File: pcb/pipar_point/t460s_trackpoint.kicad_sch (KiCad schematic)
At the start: 7 parts, among them X1 12.0 MHz

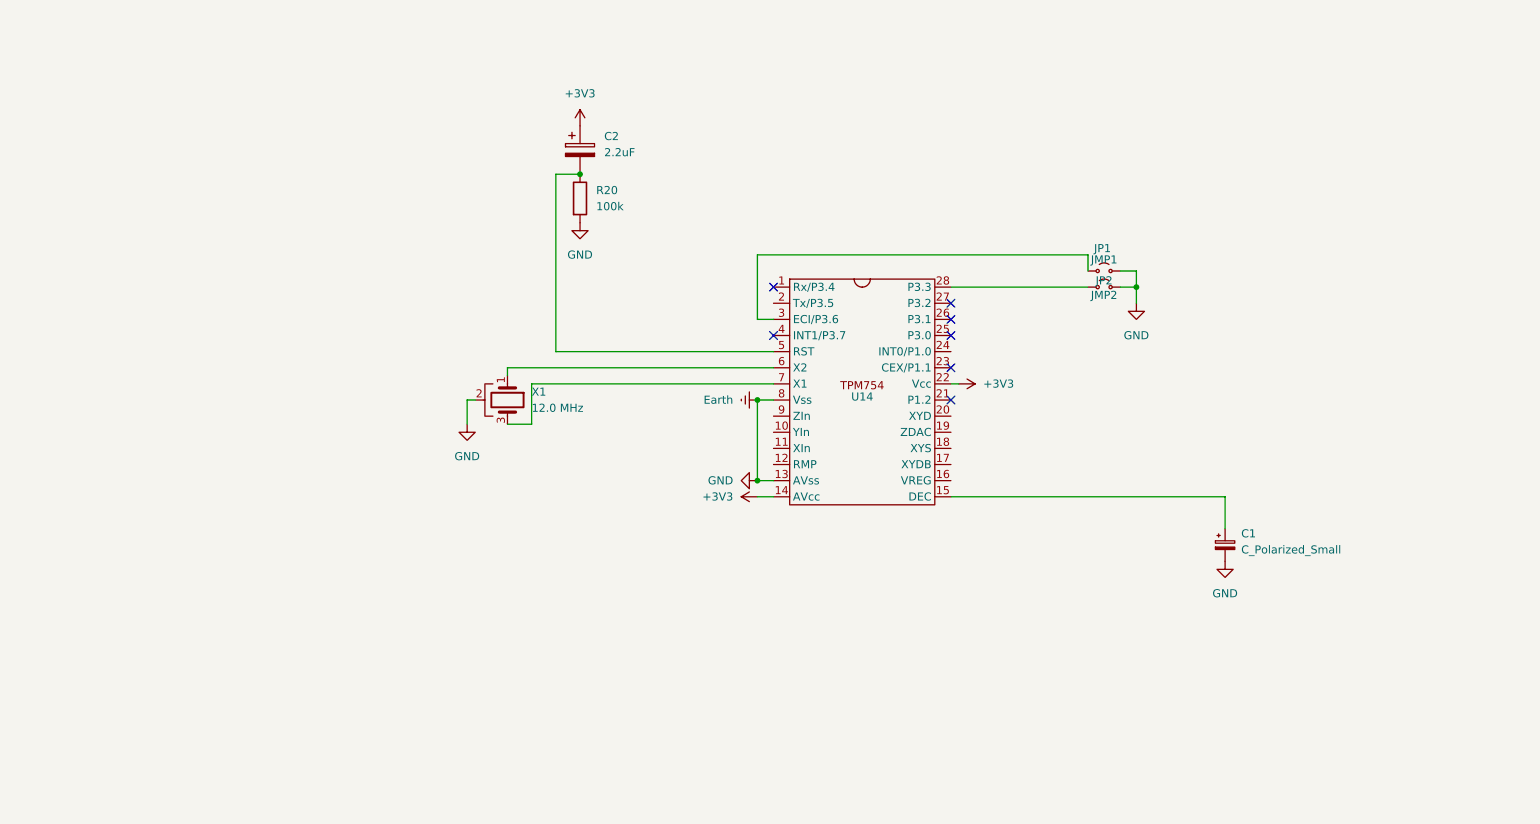
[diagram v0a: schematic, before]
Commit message: starts work on t460s board 2
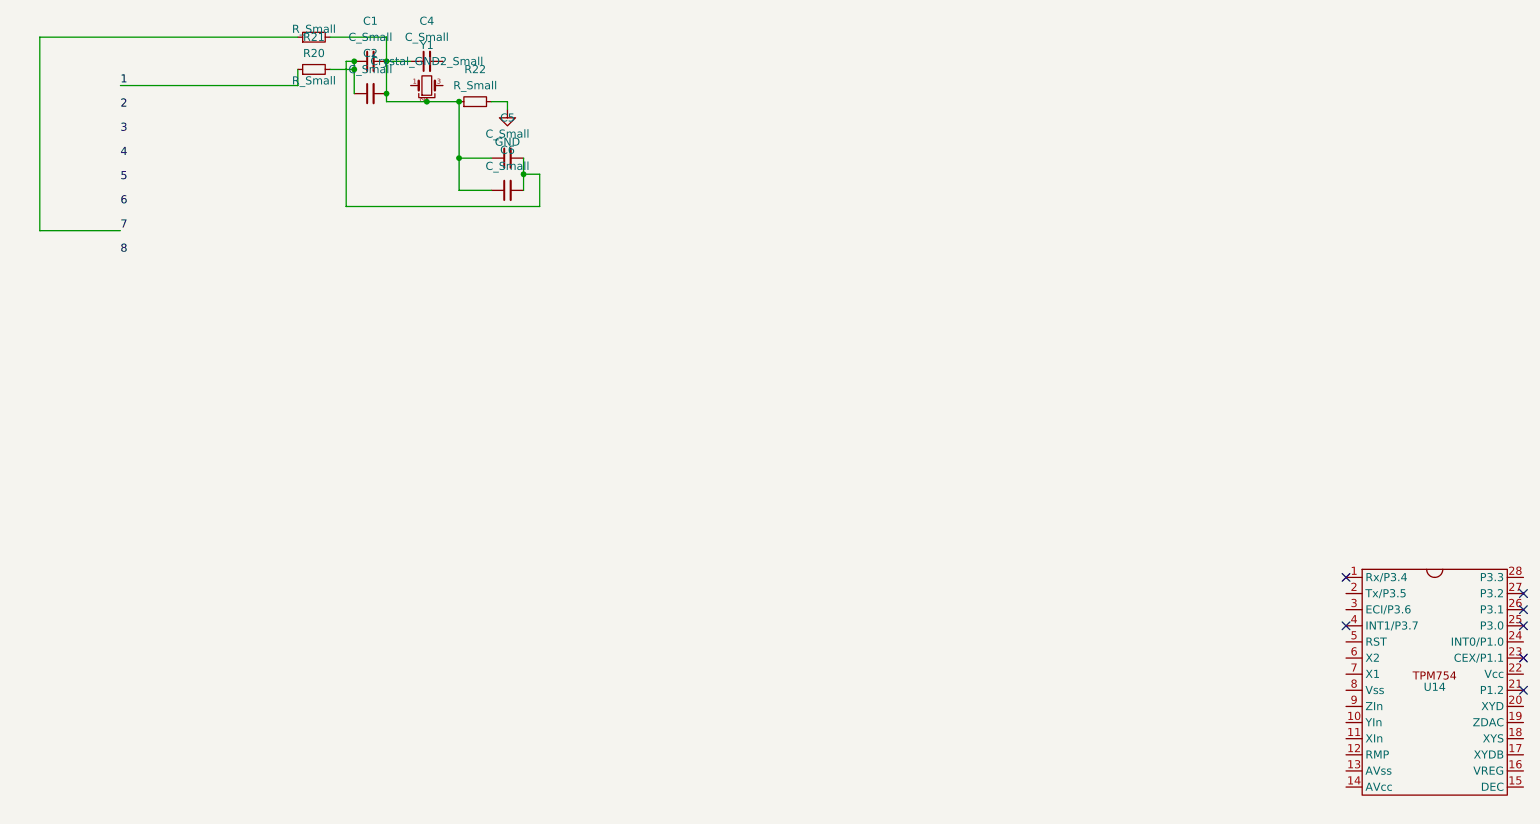
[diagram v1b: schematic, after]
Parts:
- removed C1: C_Polarized_Small, symbol Device:C_Polarized_Small
- removed C2: 2.2uF, symbol Device:C_Polarized
- removed JP1: JMP1, symbol Jumper:Jumper_2_Small_Open
- removed JP2: JMP2, symbol Jumper:Jumper_2_Small_Open
- removed R20: 100k, symbol Device:R
- removed X1: 12.0 MHz, symbol Device:Crystal_GND2
- added C1, C2, C4, C5, C6: C_Small, symbol Device:C_Small
- added R20, R21, R22: R_Small, symbol Device:R_Small
- added Y1: Crystal_GND2_Small, symbol Device:Crystal_GND2_Small
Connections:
- net +3V3: no longer names the net of U14.14 (AVcc)
- net +3V3: no longer U14.22 (Vcc)
- net Earth: no longer names the net of U14.13 (AVss)
- net Earth: no longer U14.8 (Vss)
- new net: C1.2, C2.2, C4.1, C5.1, C6.1, R20.2, R22.1, Y1.2
- new net: C1.1, C2.1, C5.2, C6.2, R21.2
- new net 1: R21.1
- new net 7: R20.1
- new net GND: R22.2
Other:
- moved on the sheet: U14

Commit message: push initial schema for t460s
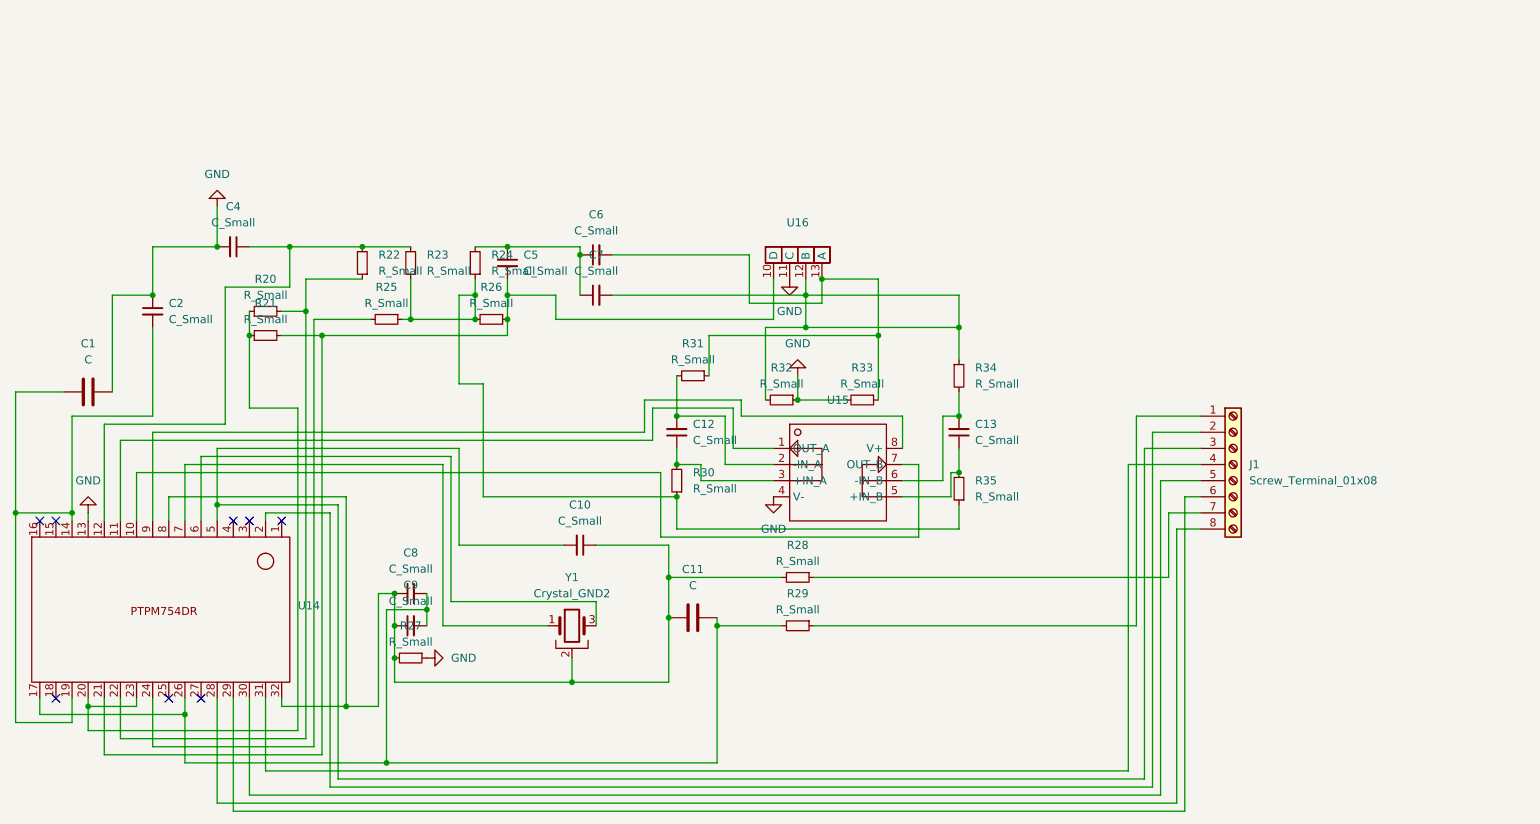
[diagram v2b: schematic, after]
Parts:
- removed C1: C_Small, symbol Device:C_Small
- removed U14: ~, symbol Trackpoint:TPM754
- removed Y1: Crystal_GND2_Small, symbol Device:Crystal_GND2_Small
- added C1, C11: C, symbol Device:C
- added C10, C12, C13, C7, C8, C9: C_Small, symbol Device:C_Small
- added J1: Screw_Terminal_01x08, symbol Connector:Screw_Terminal_01x08
- added R23, R24, R25, R26, R27, R28, R29, R30, R31, R32, R33, R34, R35: R_Small, symbol Device:R_Small
- added U14: ~, symbol Trackpoint:PTPM754DR
- added U15: ~, symbol Trackpoint:LMC6032
- added U16: ~, symbol Trackpoint:Connector
- added Y1: Crystal_GND2, symbol Device:Crystal_GND2
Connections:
- net 7 is gone; now on an unnamed net: R20.1
- net GND: now also C2.1, C4.2, C1.2, R27.1, R32.1, R33.2, U14.13, U15.4 (V-), U16.11 (C); no longer R22.2
- net at C5.2, R21.2: now also R26.1, U14.21, U16.10 (D); no longer C2.1, C6.2
- net 1: no longer names the net of R21.1
- net 1: now also U14.20, U14.23
- new net: C6.2, R31.1, R33.1, U16.13 (A)
- new net: C12.2, R31.2, U15.2 (-IN_A)
- new net: C7.2, R32.2, R34.1, U16.12 (B)
- new net: R20.2, R22.1, U14.22
- new net: C4.1, R22.2, R23.2, U14.12
- new net: R23.1, R24.1, R25.1, R26.2, R30.1, R35.1
- new net: C5.1, C6.1, C7.1, R24.2
- new net: U14.10, U15.7 (OUT_B)
- new net: U14.11, U15.1 (OUT_A)
- new net: C1.1, C2.2, U14.14, U14.19
- new net: C11.2, C8.2, C9.2, R29.2, U14.17, U14.26
- new net: J1.2 (Pin_2), U14.2
- new net: R25.2, U14.24
- new net: J1.8 (Pin_8), U14.28
- new net: J1.6 (Pin_6), U14.29
- new net: J1.5 (Pin_5), U14.30
- new net: J1.4 (Pin_4), U14.31
- new net: C10.1, C11.1, C8.1, C9.1, R27.2, R28.2, U14.32, U14.8, Y1.2
- new net: C10.2, J1.3 (Pin_3), U14.5
- new net: U14.6, Y1.3
- new net: U14.7, Y1.1
- new net: U14.9, U15.8 (V+)
- new net: J1.7 (Pin_7), R28.1
- new net: J1.1 (Pin_1), R29.1
- new net: C13.1, R35.2, U15.5 (+IN_B)
- new net: C13.2, R34.2, U15.6 (-IN_B)
- new net: C12.1, R30.2, U15.3 (+IN_A)
- no-connect marks 7 -> 8
